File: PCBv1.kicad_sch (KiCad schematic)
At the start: 14 parts, among them SW1 SW_Push, U1 ATmega32U4-A, Y1 16MHz

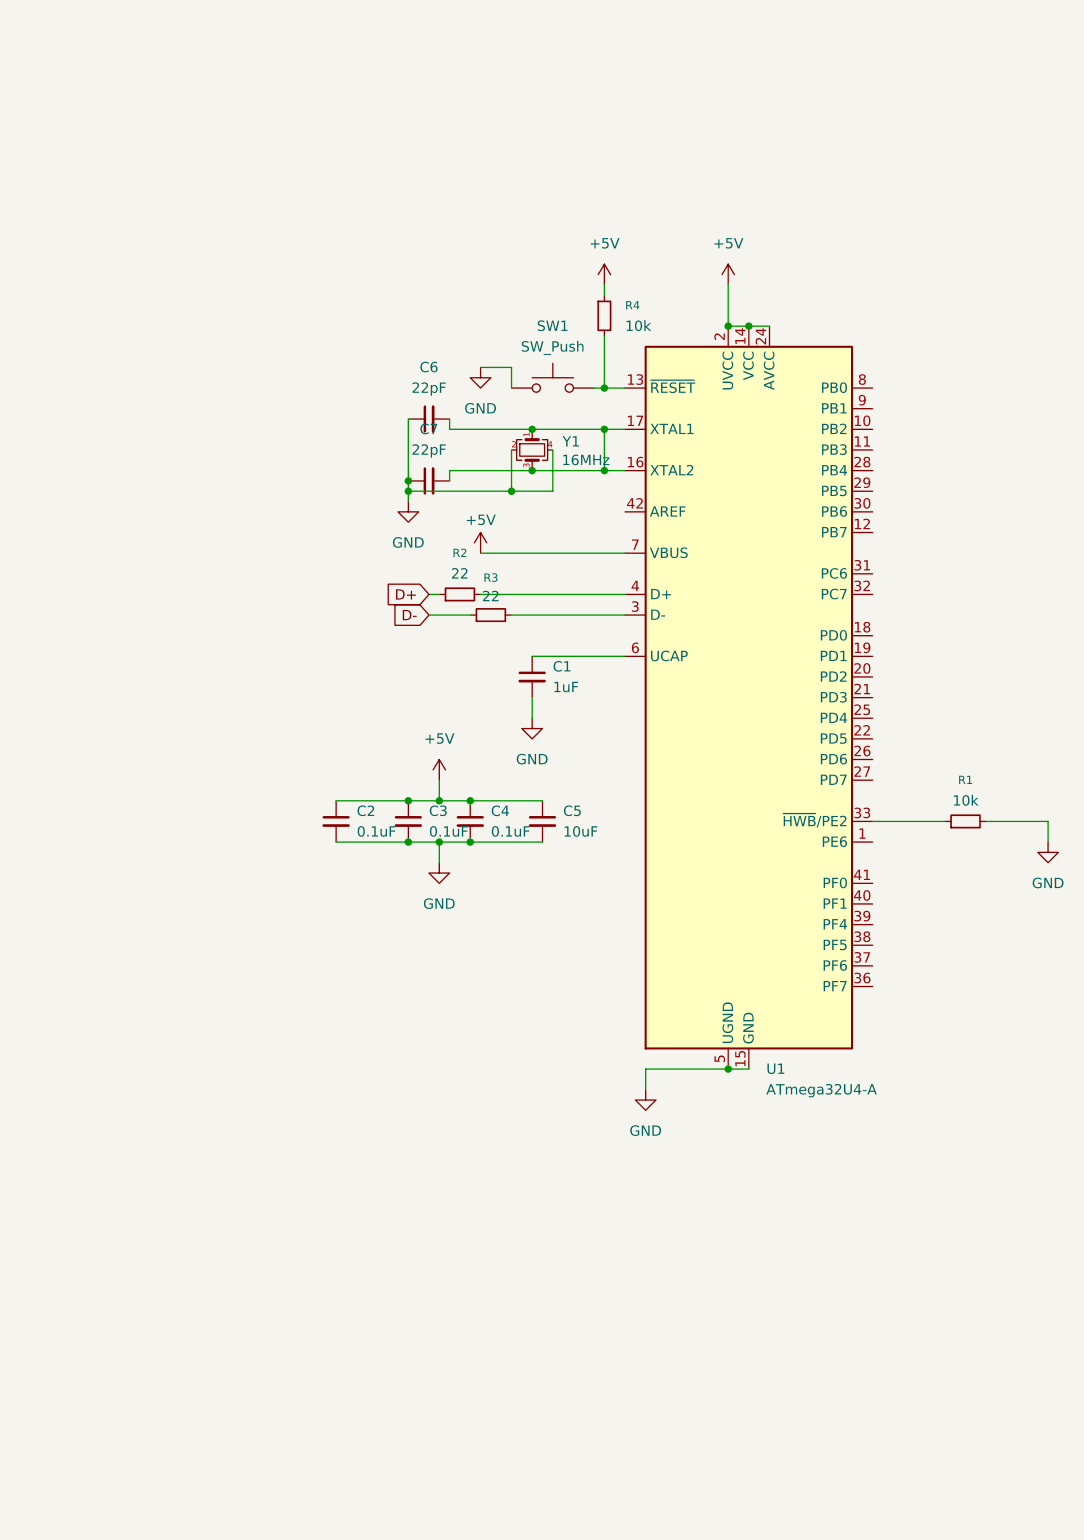
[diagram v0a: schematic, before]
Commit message: asjkdhnasjkd
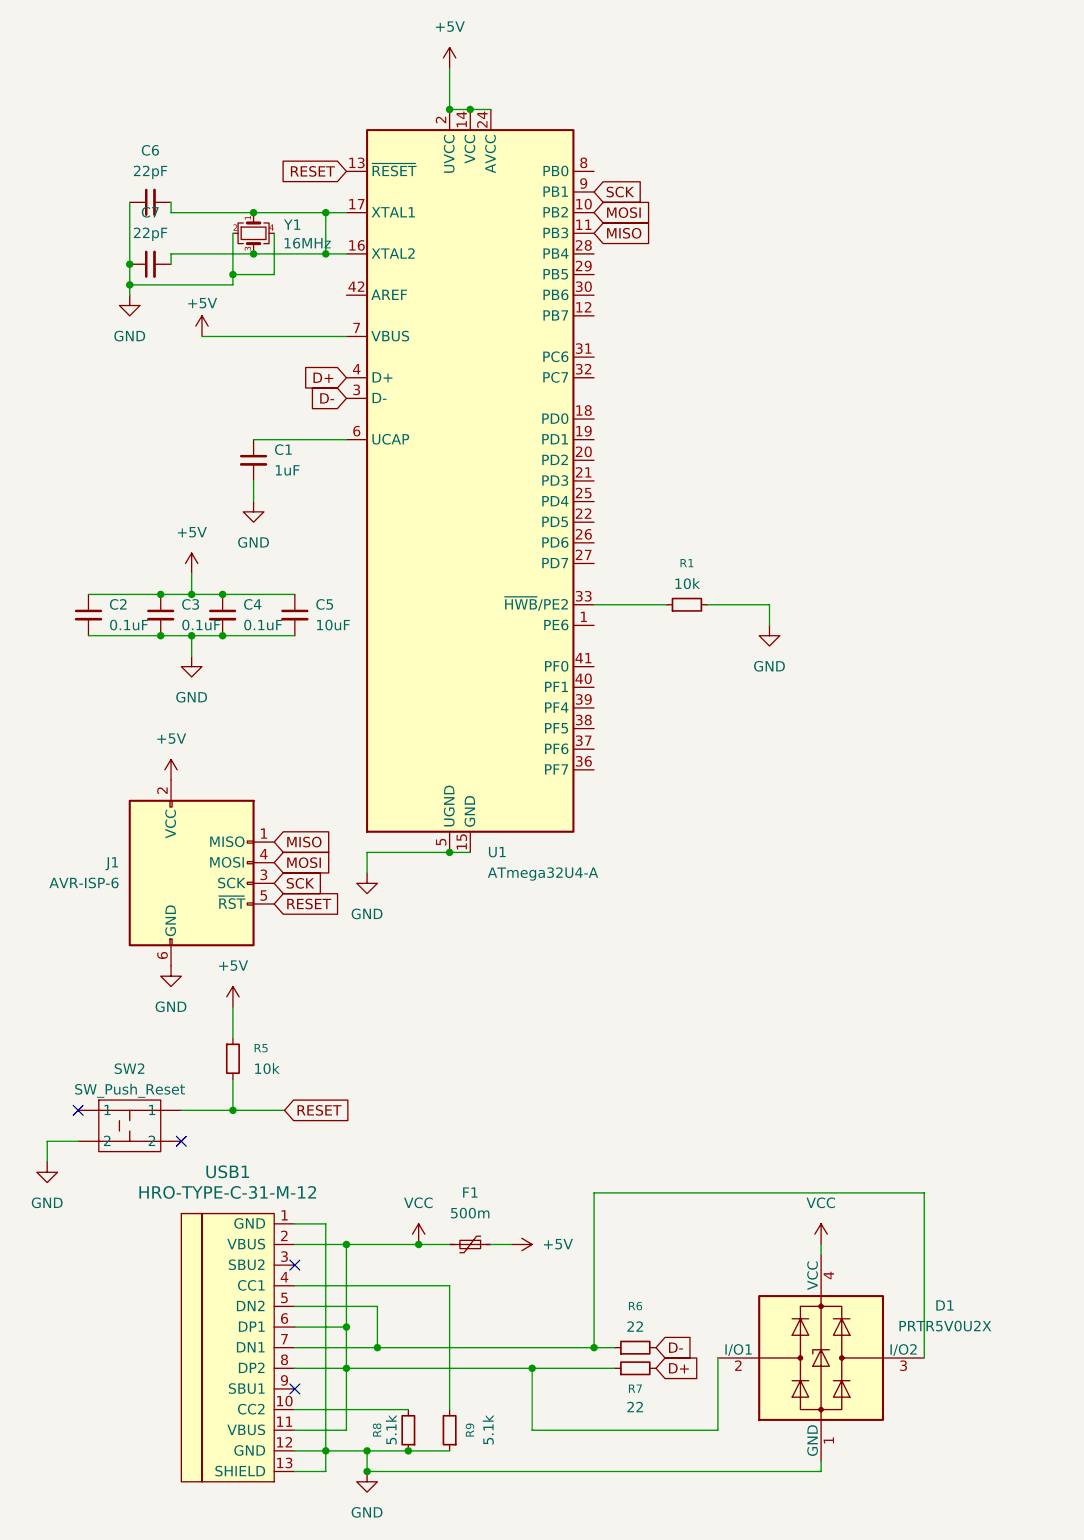
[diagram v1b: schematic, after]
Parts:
- removed R2, R3: 22, symbol Device:R_Small
- removed R4: 10k, symbol Device:R_Small
- removed SW1: SW_Push, symbol Switch:SW_Push
- added D1: PRTR5V0U2X, Package_TO_SOT_SMD:SOT-143, symbol Power_Protection:PRTR5V0U2X
- added F1: 500m, symbol Device:Polyfuse_Small
- added J1: AVR-ISP-6, symbol Connector:AVR-ISP-6
- added R5: 10k, symbol Device:R_Small
- added R6, R7: 22, symbol Device:R_Small
- added R8, R9: 5.1k, symbol Device:R_Small
- added SW2: SW_Push_Reset, symbol Local:SW_SKQG
- added USB1: HRO-TYPE-C-31-M-12, symbol Type-C:HRO-TYPE-C-31-M-12
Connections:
- net +5V: now also F1.1, J1.2 (VCC), R5.1
- net D+: now also U1.4 (D+), R7.2
- net D-: now also U1.3 (D-), R6.2
- net GND: now also D1.1 (GND), J1.6 (GND), R8.1, R9.1, SW2. (2), USB1.1 (GND), USB1.12 (GND), USB1.13 (SHIELD)
- net RESET: now reaches U1.13 (~{RESET})
- net RESET: now also J1.5 (~{RST}), R5.2, SW2. (2)
- net MOSI: now reaches U1.10 (PB2)
- net MOSI: now also J1.4 (MOSI)
- net MISO: now reaches U1.11 (PB3)
- net MISO: now also J1.1 (MISO)
- net SCK: now reaches U1.9 (PB1)
- net SCK: now also J1.3 (SCK)
- new net: R8.2, USB1.10 (CC2)
- new net: R9.2, USB1.4 (CC1)
- new net: D1.3 (I/O2), R6.1, USB1.5 (DN2), USB1.7 (DN1)
- new net VCC: D1.2 (I/O1), D1.4 (VCC), F1.2, R7.1, USB1.11 (VBUS), USB1.2 (VBUS), USB1.6 (DP1), USB1.8 (DP2)
- no-connect marks 0 -> 4
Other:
- moved on the sheet: C1, C2, C3, C4, C5, C6, C7, R1, U1, Y1
